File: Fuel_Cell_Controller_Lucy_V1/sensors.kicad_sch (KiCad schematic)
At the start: 15 parts, among them U14 MCP602-E/SN, U15 ADS1115IRUGR, U16 ADS1115IRUGR, U18 LIS3DHTR

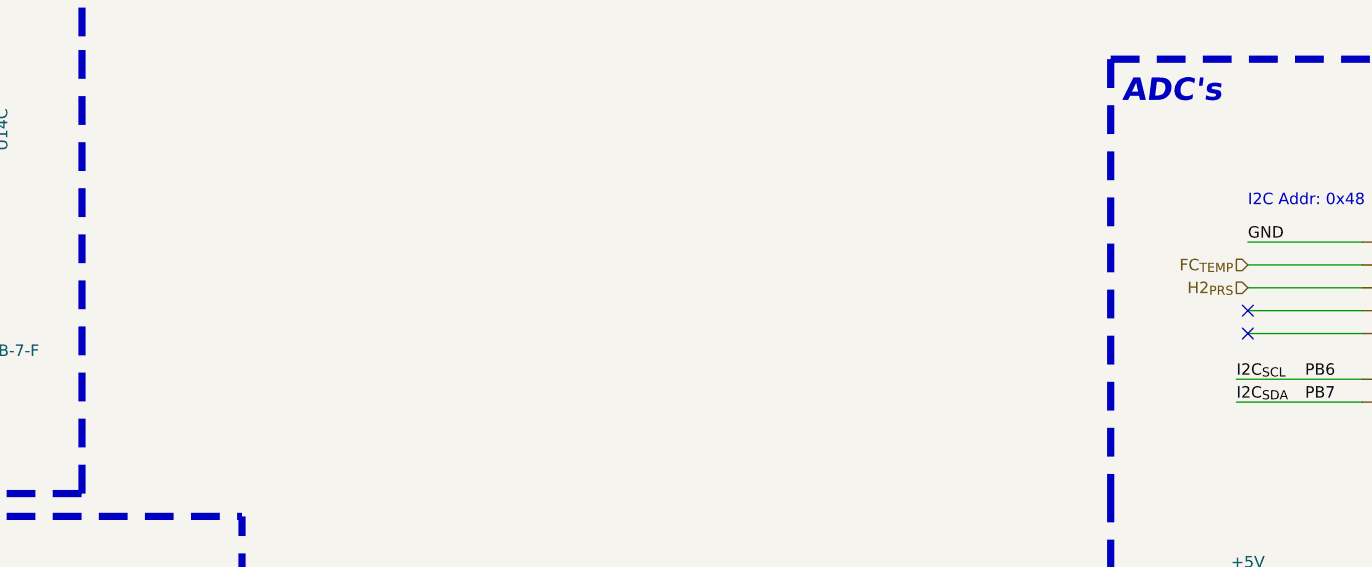
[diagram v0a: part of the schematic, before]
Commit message: $
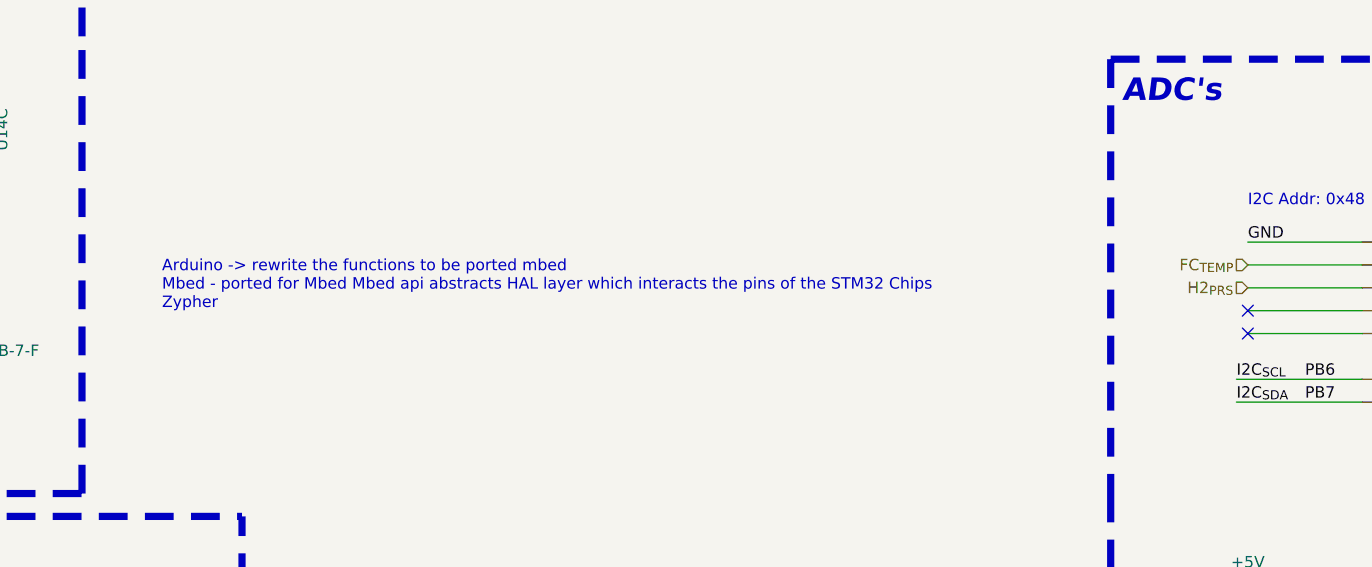
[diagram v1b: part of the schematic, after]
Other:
- note added: "Arduino -> rewrite the functions to be ported mbed Mbed - ported for Mbed Mbed api abstracts HAL layer which interacts the pins of the STM32 Chips Zypher"
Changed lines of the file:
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@@
+    (effects (font (size 1.27 1.27)) (justify left bottom))
+  )
+  (text "Arduino -> rewrite the functions to be ported mbed\nMbed - ported for Mbed Mbed api abstracts HAL layer which interacts the pins of the STM32 Chips\nZypher\n"
+    (at 97.79 92.71 0)
     (effects (font (size 1.27 1.27)) (justify left bottom))
   )
